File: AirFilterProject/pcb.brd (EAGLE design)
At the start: 100 x 81.3 mm, 18 parts, among them T1 TIP122, U1 ATMEGA328P-PU

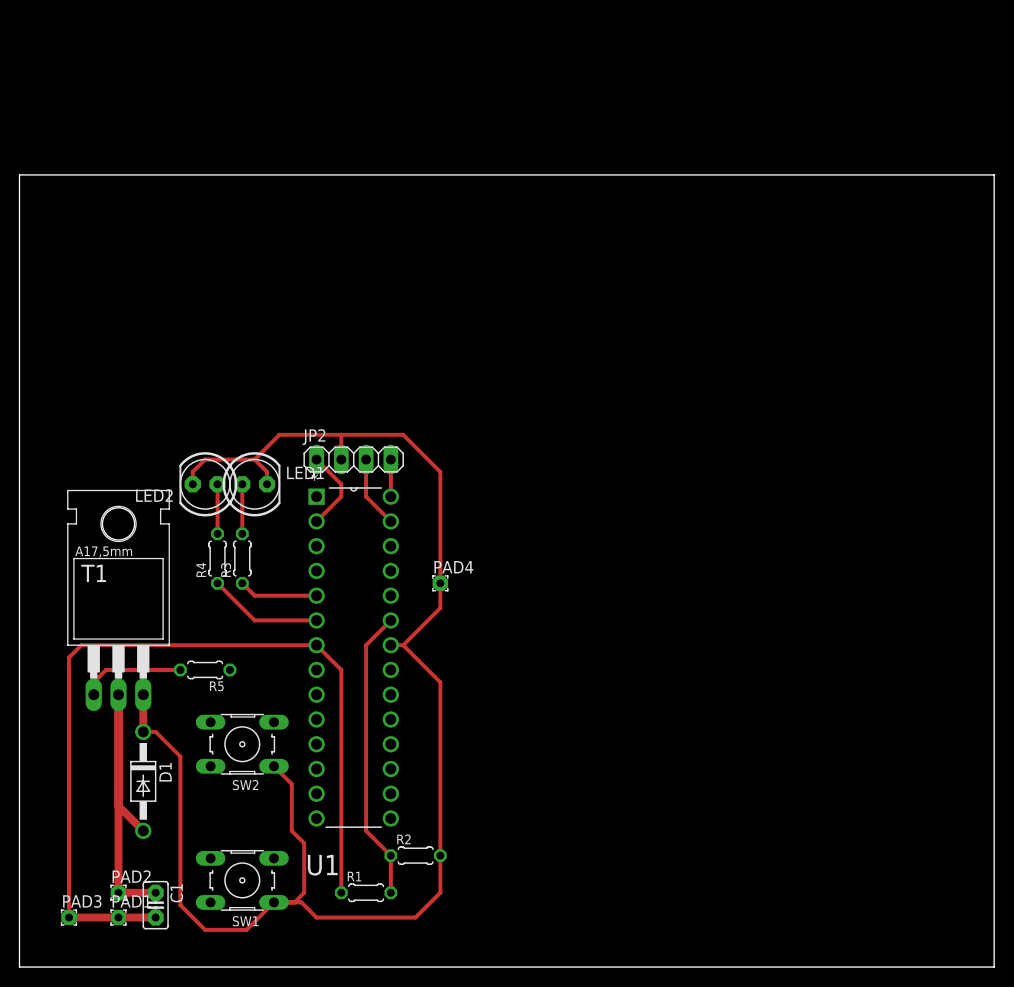
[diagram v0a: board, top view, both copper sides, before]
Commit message: Final PCB
Final Changes to PCB. Ready for printing
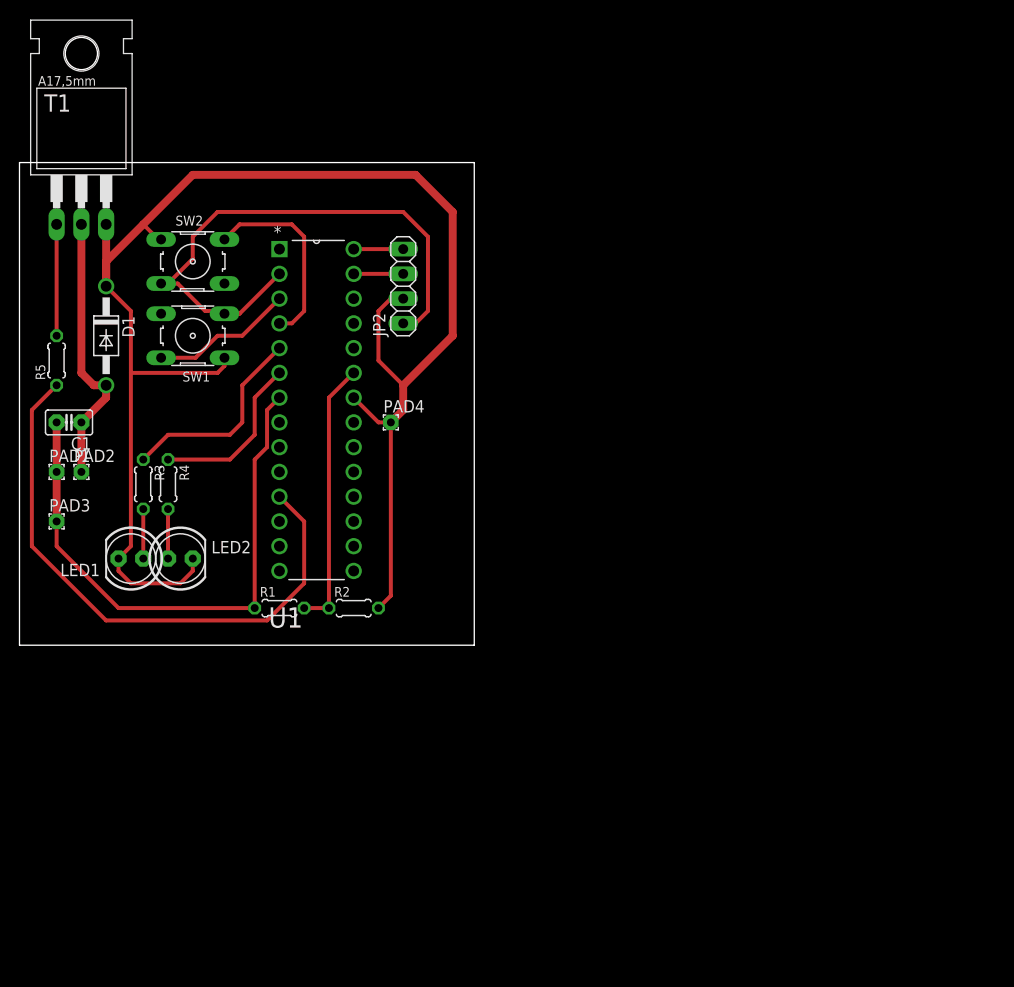
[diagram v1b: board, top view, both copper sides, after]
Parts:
- moved SW1 56.1 mm to (17.8, 63.5)
- moved C1 50.3 mm to (5.08, 54.6), turned to 180 degrees
- moved SW2 49.8 mm to (17.8, 71.1), turned to 0 degrees
- moved T1 48.4 mm to (6.35, 81.3)
- moved PAD1 46.2 mm to (3.81, 49.5)
- moved D1 45.9 mm to (8.89, 63.5)
- moved PAD2 43.3 mm to (6.35, 49.5)
- moved PAD3 40.7 mm to (3.81, 44.5)
- moved R5 35.2 mm to (3.81, 61.0), turned to 90 degrees
- moved R1 30.5 mm to (26.7, 35.6)
- moved R2 26.2 mm to (34.3, 35.6)
- moved U1 25.7 mm to (34.3, 39.4)
- moved JP2 18.5 mm to (39.4, 68.6), turned to 90 degrees
- moved PAD4 17.3 mm to (38.1, 54.6)
- moved LED1 14.8 mm to (11.4, 40.6), turned to 180 degrees
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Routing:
- net N$13: track 0.00 -> 60.2 mm
- net N$5: track 8.45 -> 57.9 mm
- net N$7: track 0.00 -> 20.0 mm
- net VCC: track 87.9 -> 68.5 mm
- net N$6: track 0.00 -> 14.7 mm
- net N$8: track 8.15 -> 20.9 mm
- net N$2: track 39.2 -> 28.2 mm
- net GND: track 155.3 -> 164.0 mm
- net N$9: track 11.7 -> 17.3 mm
- net N$4: track 30.0 -> 27.7 mm
- net N$1: track 7.40 -> 5.08 mm
- net N$3: track 3.81 -> 5.08 mm
- net N$12: track 10.7 -> 11.4 mm
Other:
- board size 100 x 81.3 mm -> 46.7 x 49.5 mm
